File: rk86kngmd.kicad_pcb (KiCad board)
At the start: 2 copper layers, 86.9 x 84.7 mm, 32 parts, among them J1 Conn_02x17_Odd_Even, J2 FD power, X1 ОНп-КС-23

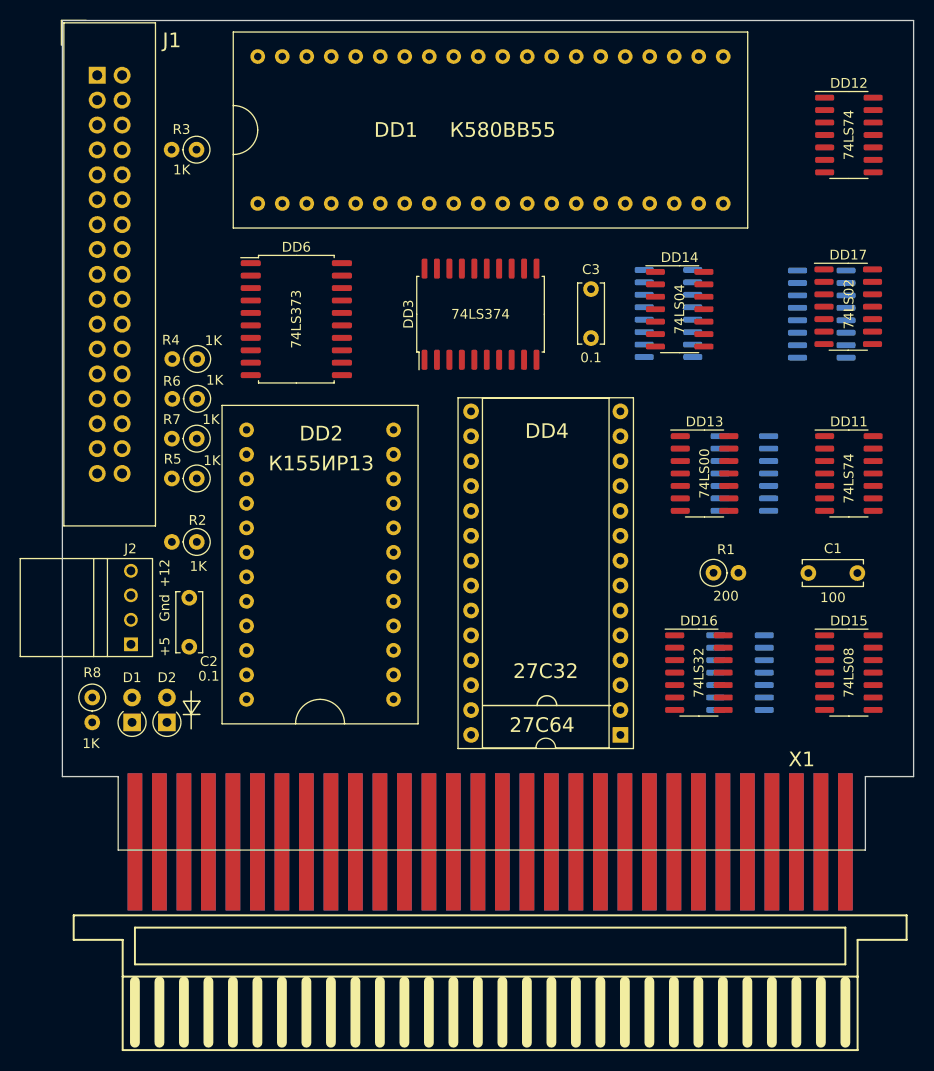
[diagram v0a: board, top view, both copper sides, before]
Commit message: board routed
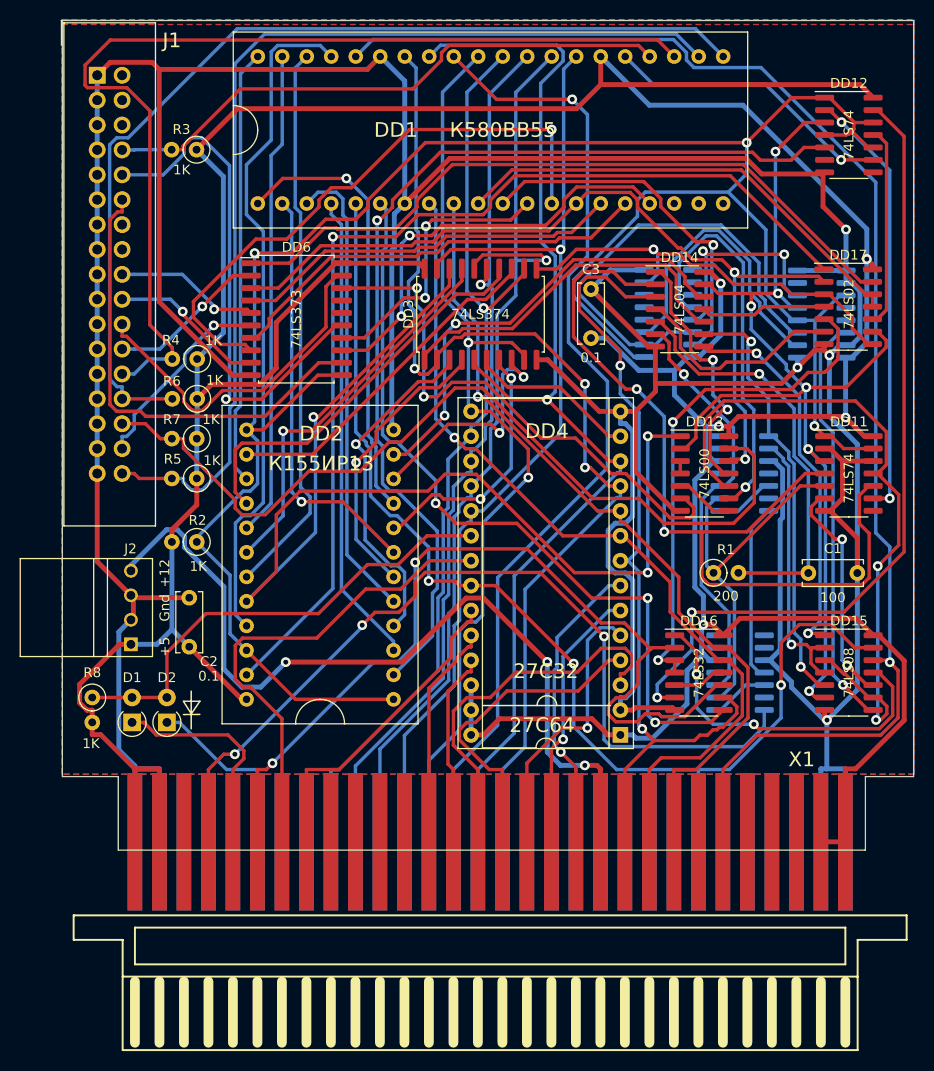
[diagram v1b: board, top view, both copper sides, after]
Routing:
- net GND: track 0.00 -> 498.6 mm, vias 0 -> 4
- net +5V: track 0.00 -> 427.5 mm, vias 0 -> 5
- net Net-(DD10-Pad1): track 0.00 -> 231.3 mm, vias 0 -> 3
- net /WR: track 0.00 -> 145.1 mm, vias 0 -> 1
- net /RD: track 0.00 -> 118.1 mm, vias 0 -> 3
- net /D2: track 0.00 -> 117.9 mm, vias 0 -> 1
- net /D1: track 0.00 -> 116.4 mm, vias 0 -> 1
- net Net-(DD13-Pad1): track 0.00 -> 114.1 mm, vias 0 -> 3
- net /D0: track 0.00 -> 109.6 mm, vias 0 -> 3
- net Net-(DD11-Pad3): track 0.00 -> 108.8 mm, vias 0 -> 6
- net Net-(DD17-Pad1): track 0.00 -> 105.4 mm, vias 0 -> 1
- net TR00: track 0.00 -> 103.7 mm
- net READY: track 0.00 -> 103.5 mm
- net /D7: track 0.00 -> 102.0 mm, vias 0 -> 1
- net Net-(DD12-Pad5): track 0.00 -> 101.1 mm, vias 0 -> 1
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- added copper zone on B.Cu, net GND
- added copper zone on F.Cu, net GND
